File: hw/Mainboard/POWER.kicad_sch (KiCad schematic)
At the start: 63 parts, among them J1 9V POWER, J2 9V POWER, J3 PET POWER, J4 5V PWR, U3 LM317AG-TN3-R, U4 XL1509-5.0E1, U5 LM317AG-TN3-R, U6 AMS1117-3.3

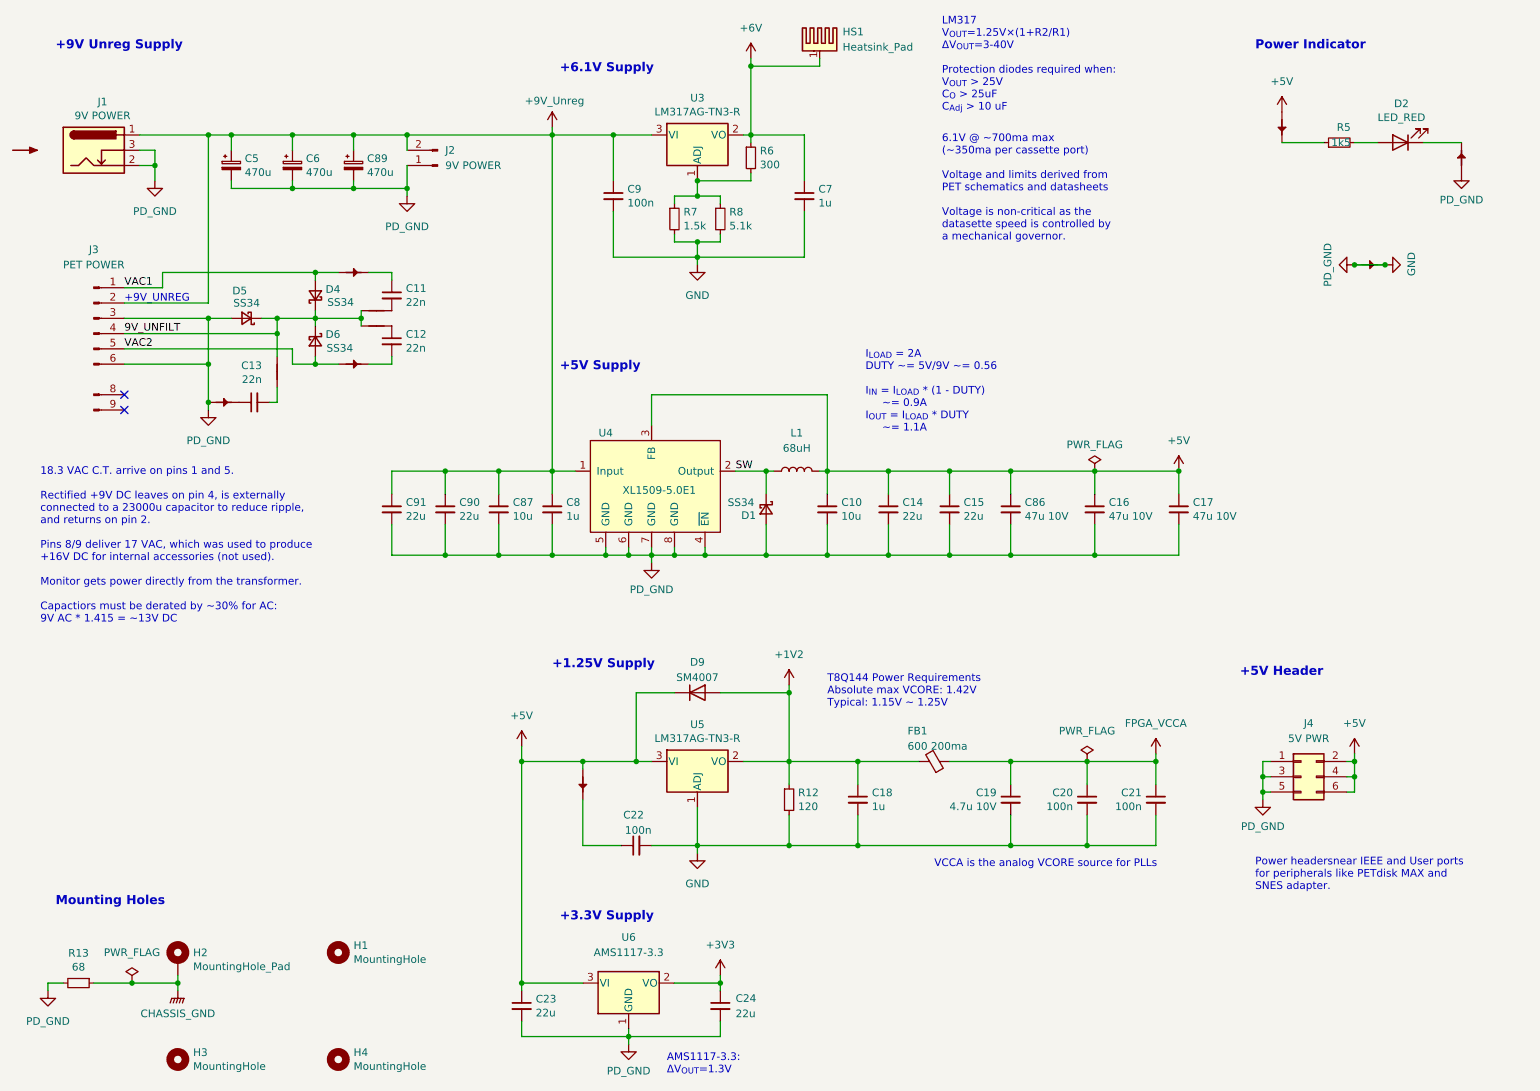
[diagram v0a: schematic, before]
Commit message: hw: fill, routing, and silk touchups (wip)
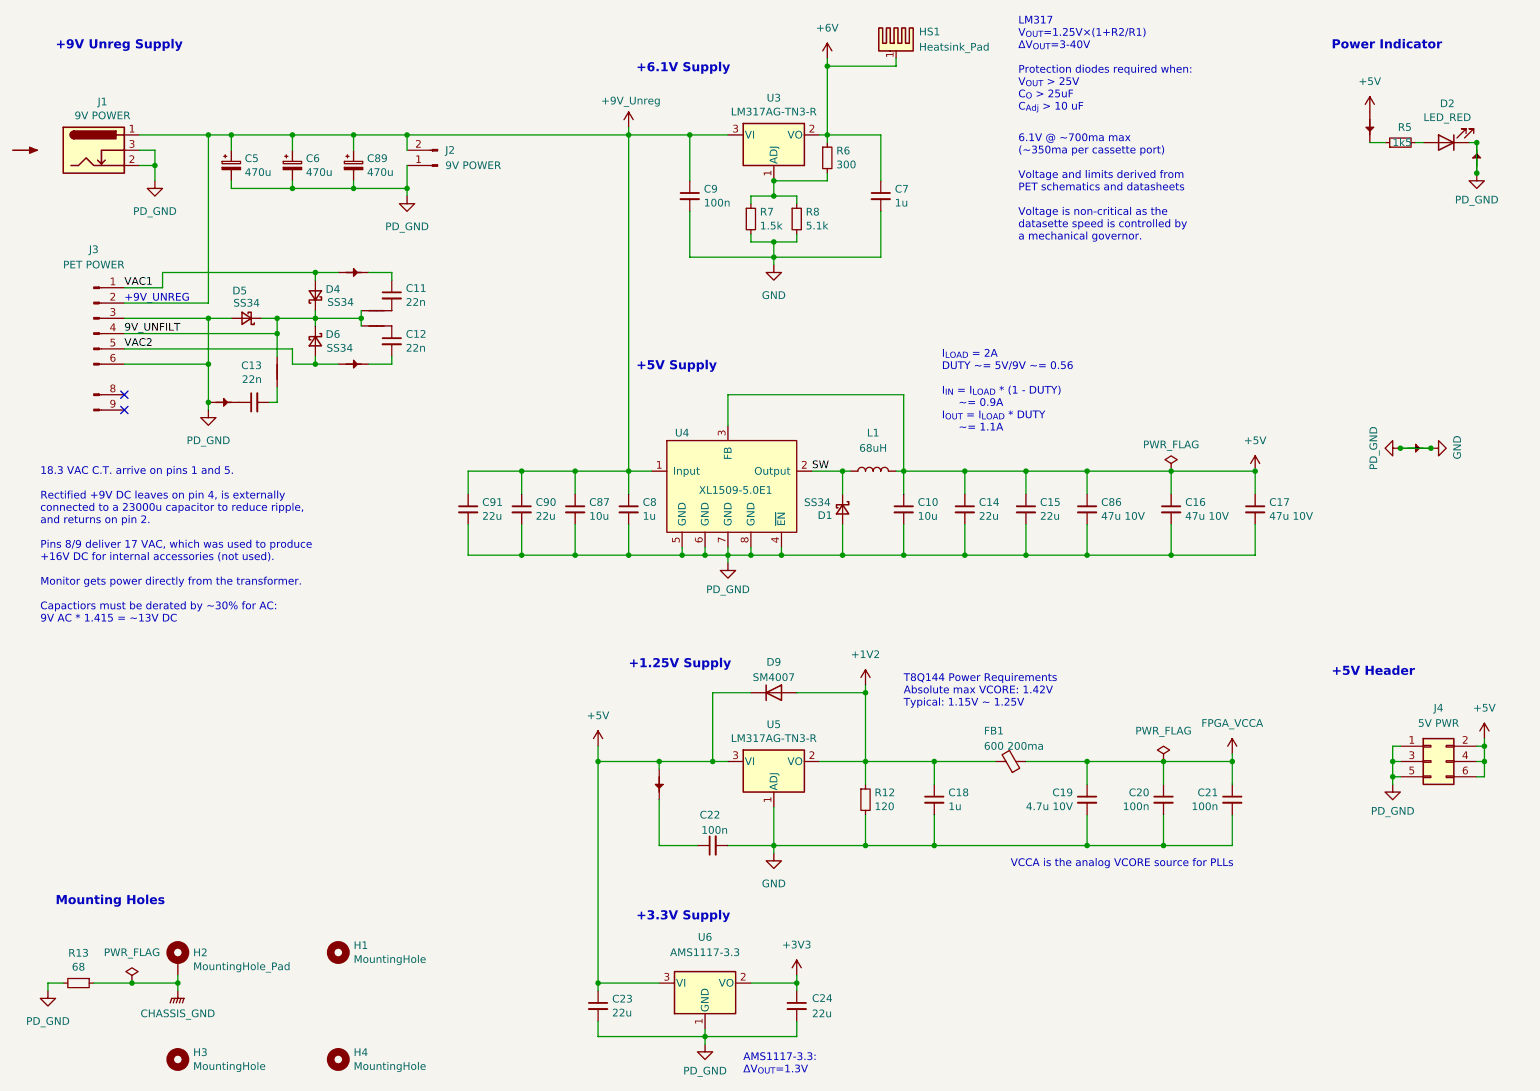
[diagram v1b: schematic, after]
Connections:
- net GND: now also D2.1 (K), PT4.2
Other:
- note removed: "Power headersnear IEEE and User ports for peripherals like PETdisk MAX and SNES adapter."
- moved on the sheet: C10, C14, C15, C16, C17, C18, C19, C20, C21, C22, C23, C24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
